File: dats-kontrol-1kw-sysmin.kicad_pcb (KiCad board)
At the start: 2 copper layers, 26 parts, among them J1 SWD, J2 Conn_01x12, J3 USB_B, SW1 SW?, U1 AMS1117CD-3.3, U2 STM32F4X1CXU6, Y1 25MHZ 9PF, Y2 32.768KHz

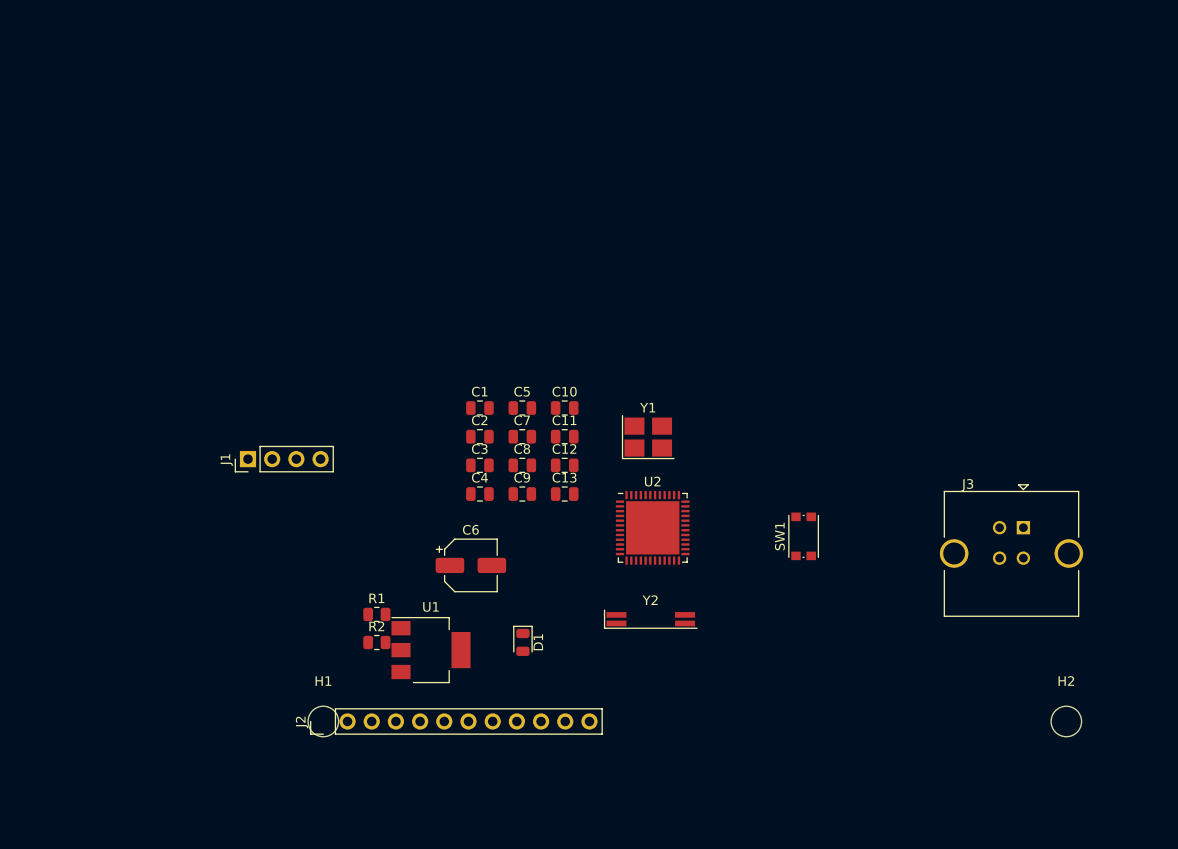
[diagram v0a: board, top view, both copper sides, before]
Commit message: new layout
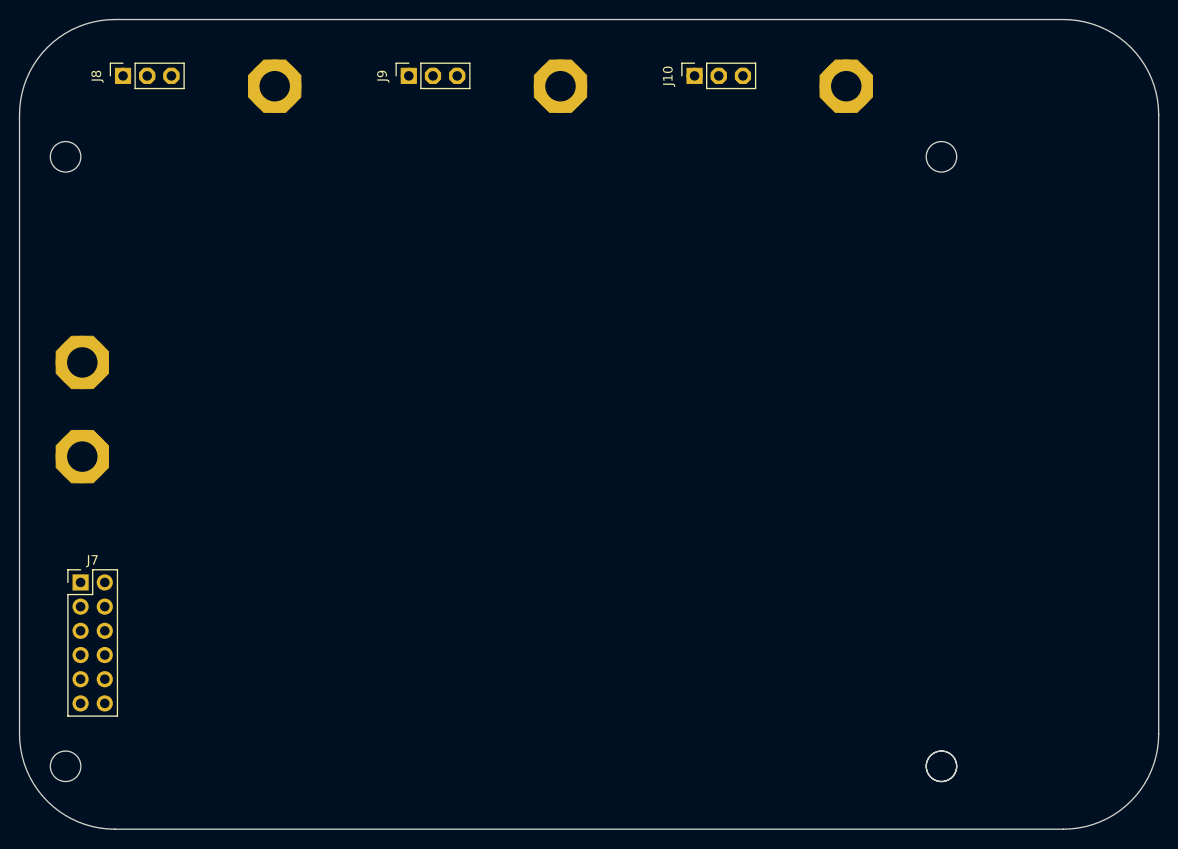
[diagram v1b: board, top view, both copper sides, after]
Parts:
- removed C1: 10uF, Capacitor_SMD:C_0805_2012Metric
- removed C10, C11, C12, C9: 100nF, Capacitor_SMD:C_0805_2012Metric
- removed C13: 100 nF, Capacitor_SMD:C_0805_2012Metric
- removed C2, C3: 12pF, Capacitor_SMD:C_0805_2012Metric
- removed C4, C5, C8: 4.3pF, Capacitor_SMD:C_0805_2012Metric
- removed C6: 10 uF, Capacitor_SMD:CP_Elec_5x5.3
- removed C7: 22 uF, Capacitor_SMD:C_0805_2012Metric
- removed D1: LED, LED_SMD:LED_0805_2012Metric
- removed H1, H2: M3_MH, MountingHole:MountingHole_3.2mm_M3
- removed J1: SWD, Connector_PinHeader_2.54mm:PinHeader_1x04_P2.54mm_Vertical
- removed J2: Conn_01x12, Connector_PinHeader_2.54mm:PinHeader_1x12_P2.54mm_Vertical
- removed J3: USB_B, Connector_USB:USB_B_TE_5787834_Vertical
- removed R1: 10, Resistor_SMD:R_0805_2012Metric
- removed R2: 10K, Resistor_SMD:R_0805_2012Metric
- removed SW1: SW?, Button_Switch_SMD:SW_Push_1P1T_NO_CK_KMR2
- removed U1: AMS1117CD-3.3, Package_TO_SOT_SMD:SOT-223-3_TabPin2
- removed U2: STM32F4X1CXU6, Package_DFN_QFN:QFN-48-1EP_7x7mm_P0.5mm_EP5.6x5.6mm
- removed Y1: 25MHZ 9PF, Crystal:Crystal_SMD_3225-4Pin_3.2x2.5mm_HandSoldering
- removed Y2: 32.768KHz, Crystal:Crystal_SMD_SeikoEpson_MC146-4Pin_6.7x1.5mm_HandSoldering
- added ?: , , F.Cu at (187.9, 70.8)
- added ?: , , F.Cu at (107.7, 99.8)
- added ?: MountingHole_3.2mm_M3, MountingHole:MountingHole_3.2mm_M3, F.Cu at (105.9, 78.3)
- added ?: MountingHole_3.2mm_M3, MountingHole:MountingHole_3.2mm_M3, F.Cu at (197.9, 142.2)
- added ?: MountingHole_3.2mm_M3, MountingHole:MountingHole_3.2mm_M3, F.Cu at (197.9, 78.3)
- added ?: , , F.Cu at (127.9, 70.8)
- added ?: , , F.Cu at (157.9, 70.8)
- added ?: MountingHole_3.2mm_M3, MountingHole:MountingHole_3.2mm_M3, F.Cu at (105.9, 142.2)
- added ?: , , F.Cu at (197.9, 142.2)
- added ?: , , F.Cu at (107.7, 109.7)
- added J10: PHASE_C_ISENSE, Connector_PinSocket_2.54mm:PinSocket_1x03_P2.54mm_Vertical, F.Cu at (171.9, 69.8)
- added J7: Conn_01x12, Connector_PinHeader_2.54mm:PinHeader_2x06_P2.54mm_Vertical, F.Cu at (107.5, 122.9)
- added J8: PHASE_A_ISENSE, Connector_PinSocket_2.54mm:PinSocket_1x03_P2.54mm_Vertical, F.Cu at (111.9, 69.8)
- added J9: PHASE_B_ISENSE, Connector_PinSocket_2.54mm:PinSocket_1x03_P2.54mm_Vertical, F.Cu at (141.9, 69.8)
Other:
- board outline added: 119.6 x 85 mm
